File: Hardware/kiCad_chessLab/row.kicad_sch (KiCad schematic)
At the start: 2 parts, among them U4 74HC4051

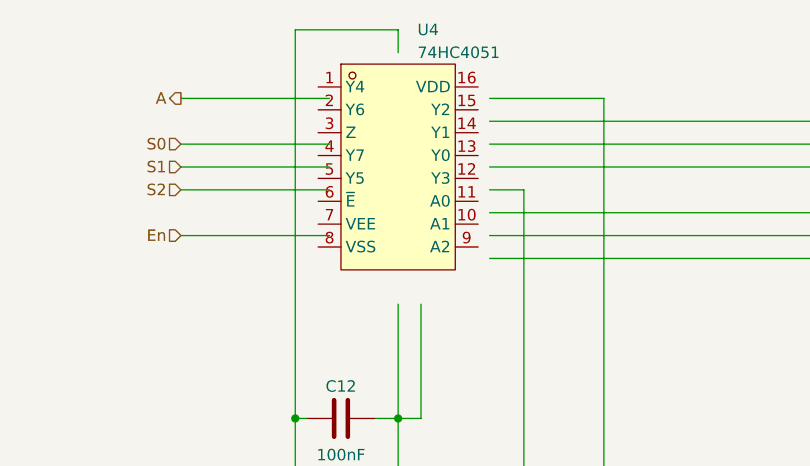
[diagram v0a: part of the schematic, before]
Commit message: Usb c new design
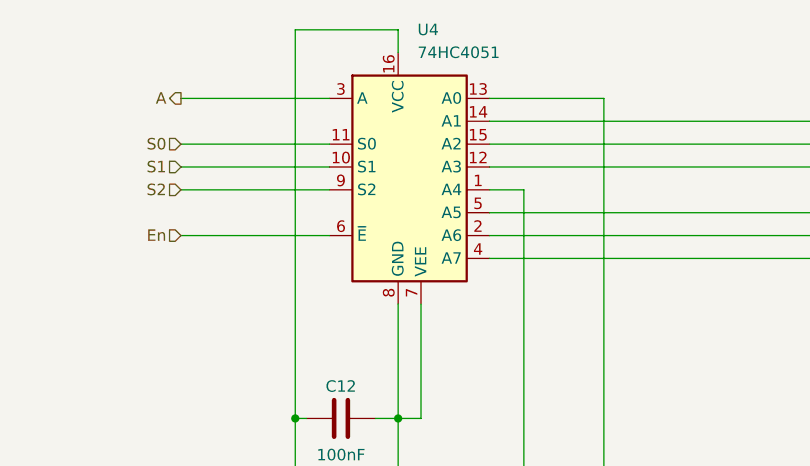
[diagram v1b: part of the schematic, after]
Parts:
- U4: footprint chessLab-footprints:SOP-16_L9.9-W3.9-P1.27-LS6.0-BL -> chessLab-footprints:74HC4051D653; symbol chessLab-symbols:74HC4051DRG -> 74xx:74HC4051
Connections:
- net A: now also U4.3 (A)
- net En: now also U4.6 (~{E})
- net GND: now also U4.7 (VEE), U4.8 (GND)
- net S0: now also U4.11 (S0)
- net S1: now also U4.10 (S1)
- net S2: now also U4.9 (S2)
- net VCC_3V3: now also U4.16 (VCC)
- net cell_B1/SIG: now also U4.13 (A0)
- net cell_B2/SIG: now also U4.14 (A1)
- net cell_B3/SIG: now also U4.15 (A2)
- net cell_B4/SIG: now also U4.12 (A3)
- net cell_B5/SIG: now also U4.1 (A4)
- net cell_B6/SIG: now also U4.5 (A5)
- net cell_B7/SIG: now also U4.2 (A6)
- net cell_B8/SIG: now also U4.4 (A7)
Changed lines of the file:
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@@
 	)
 	(symbol
-		(lib_id "chessLab-symbols:74HC4051DRG")
+		(lib_id "74xx:74HC4051")
 		(at 92.71 50.8 0)
 		(unit 1)
@@
 			)
 		)
-		(property "Footprint" "chessLab-footprints:SOP-16_L9.9-W3.9-P1.27-LS6.0-BL"
+		(property "Footprint" "chessLab-footprints:74HC4051D653"
 			(at 92.71 60.96 0)
 			(hide yes)

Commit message: NEW REFERENCES
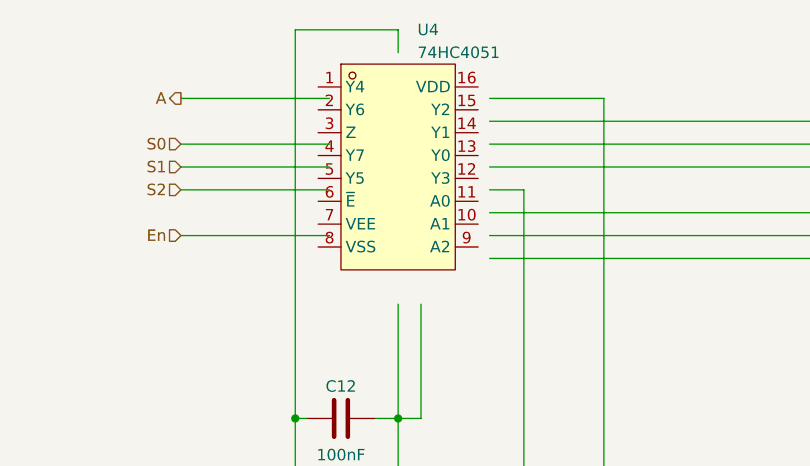
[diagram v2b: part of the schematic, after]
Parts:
- U4: footprint chessLab-footprints:74HC4051D653 -> chessLab-footprints:SOP-16_L9.9-W3.9-P1.27-LS6.0-BL; symbol 74xx:74HC4051 -> chessLab-symbols:74HC4051DRG
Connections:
- net A: no longer U4.3 (A)
- net En: no longer U4.6 (~{E})
- net GND: no longer U4.7 (VEE), U4.8 (GND)
- net S0: no longer U4.11 (S0)
- net S1: no longer U4.10 (S1)
- net S2: no longer U4.9 (S2)
- net VCC_3V3: no longer U4.16 (VCC)
- net cell_B1/SIG: no longer U4.13 (A0)
- net cell_B2/SIG: no longer U4.14 (A1)
- net cell_B3/SIG: no longer U4.15 (A2)
- net cell_B4/SIG: no longer U4.12 (A3)
- net cell_B5/SIG: no longer U4.1 (A4)
- net cell_B6/SIG: no longer U4.5 (A5)
- net cell_B7/SIG: no longer U4.2 (A6)
- net cell_B8/SIG: no longer U4.4 (A7)
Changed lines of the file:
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@@
 	)
 	(symbol
-		(lib_id "74xx:74HC4051")
+		(lib_id "chessLab-symbols:74HC4051DRG")
 		(at 92.71 50.8 0)
 		(unit 1)
@@
 			)
 		)
-		(property "Footprint" "chessLab-footprints:74HC4051D653"
+		(property "Footprint" "chessLab-footprints:SOP-16_L9.9-W3.9-P1.27-LS6.0-BL"
 			(at 92.71 60.96 0)
 			(hide yes)
